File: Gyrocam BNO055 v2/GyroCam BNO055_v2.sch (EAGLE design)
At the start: 24 parts, among them IC1 STM32G070KBT6

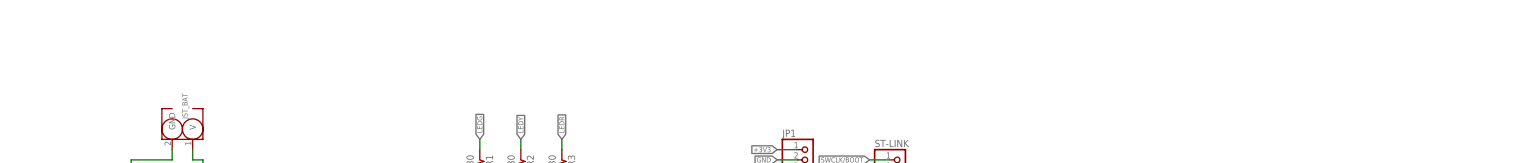
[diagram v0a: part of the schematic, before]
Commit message: Add files via upload
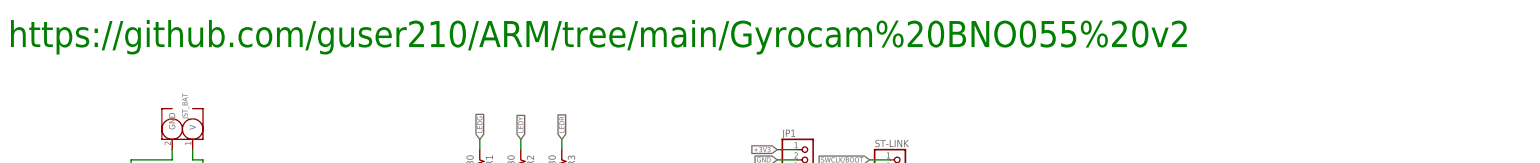
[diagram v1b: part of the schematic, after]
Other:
- note added: "https://github.com/guser210/ARM/tree/main/Gyrocam%20BNO055%20v2"
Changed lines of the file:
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@@
 <sheet>
 <plain>
+<text x="-50.8" y="177.8" size="6.4516" layer="91" ratio="12">https://github.com/guser210/ARM/tree/main/Gyrocam%20BNO055%20v2</text>
 </plain>
 <instances>
